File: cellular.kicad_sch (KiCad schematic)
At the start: 48 parts, among them J2 SIM_Card, J4 SIM_Card, Q2 BC847, U10 SMF15CT1G, U11 SN74AXC4T245PWR, U5 SMF15CT1G

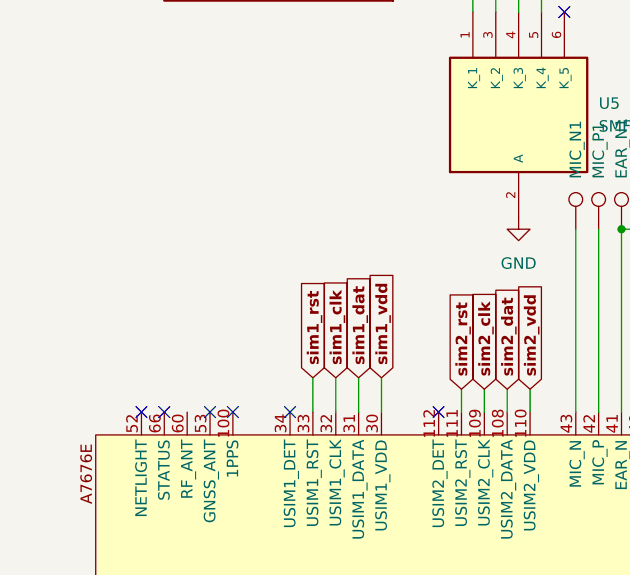
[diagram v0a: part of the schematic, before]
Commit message: lol
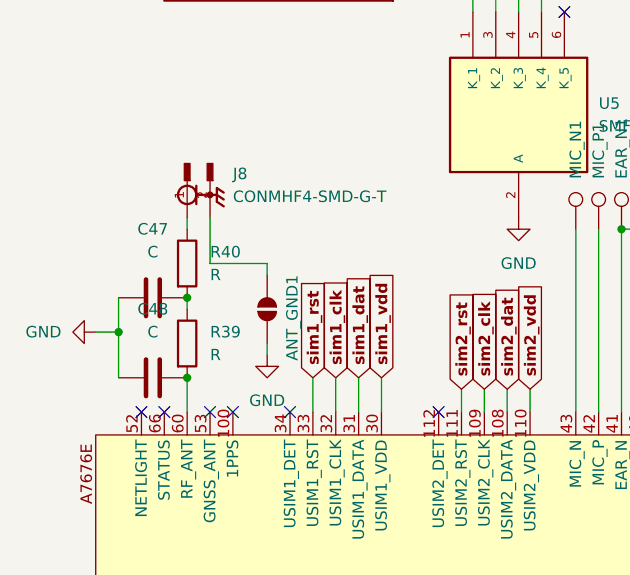
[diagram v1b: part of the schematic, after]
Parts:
- added ANT_GND1: SolderJumper_2_Open, Jumper:SolderJumper-2_P1.3mm_Open_Pad1.0x1.5mm, symbol Jumper:SolderJumper_2_Open
- added C47, C48: C, Capacitor_SMD:C_0603_1608Metric_Pad1.08x0.95mm_HandSolder, symbol Device:C
- added J8: CONMHF4-SMD-G-T, CONMHF4-SMD-G-T:TE_CONMHF4-SMD-G-T, symbol CONMHF4-SMD-G-T:CONMHF4-SMD-G-T
- added R39, R40: R, Resistor_SMD:R_0603_1608Metric_Pad0.98x0.95mm_HandSolder, symbol Device:R
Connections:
- net GND: now also ANT_GND1.1 (A), C47.1, C48.1
- net at U9.60 (RF_ANT): now also C48.2, R39.2
- new net: J8.1, R40.1
- new net: ANT_GND1.2 (B), J8.2, J8.3, J8.4
- new net: C47.2, R39.1, R40.2
